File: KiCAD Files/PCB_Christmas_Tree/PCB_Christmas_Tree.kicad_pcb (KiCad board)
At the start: 2 copper layers, 129.4 x 60.1 mm, 67 parts, among them J1 Conn_01x03_Pin, J2 CR2032, J3 Conn_01x04_Pin, J4 Conn_01x04_Pin, J5 Conn_01x04_Pin, J7 Conn_01x04_Pin, Q1 PMOS, Q2 PMOS, Q3 PMOS, Q4 NPN, Q5 PMOS, SW1 SW_Omron_B3FS, U1 ATtiny402-SS

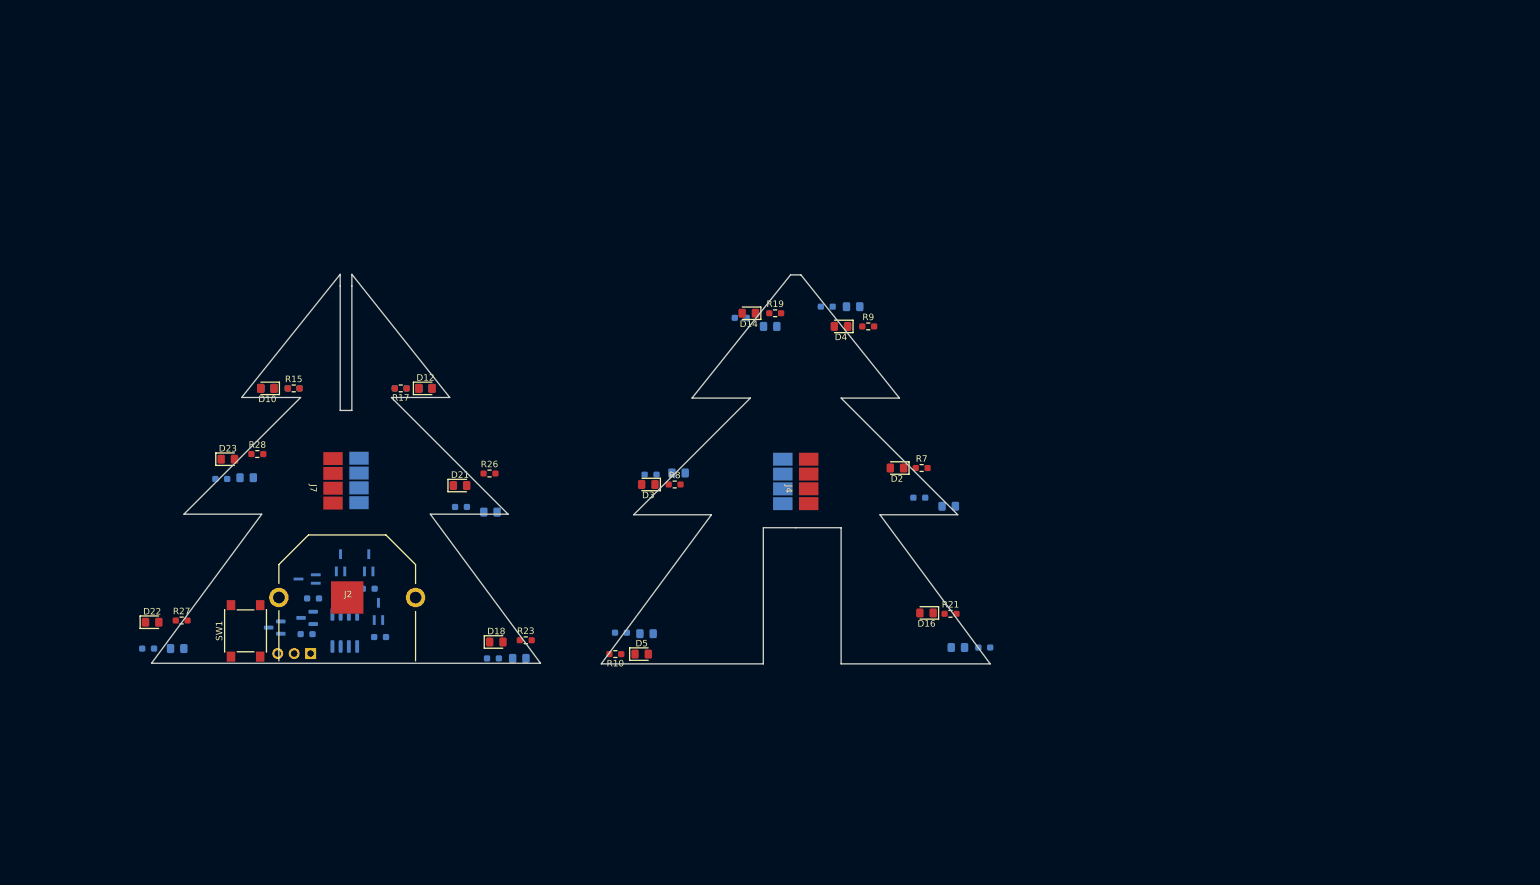
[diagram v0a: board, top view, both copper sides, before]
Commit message: pcb revision
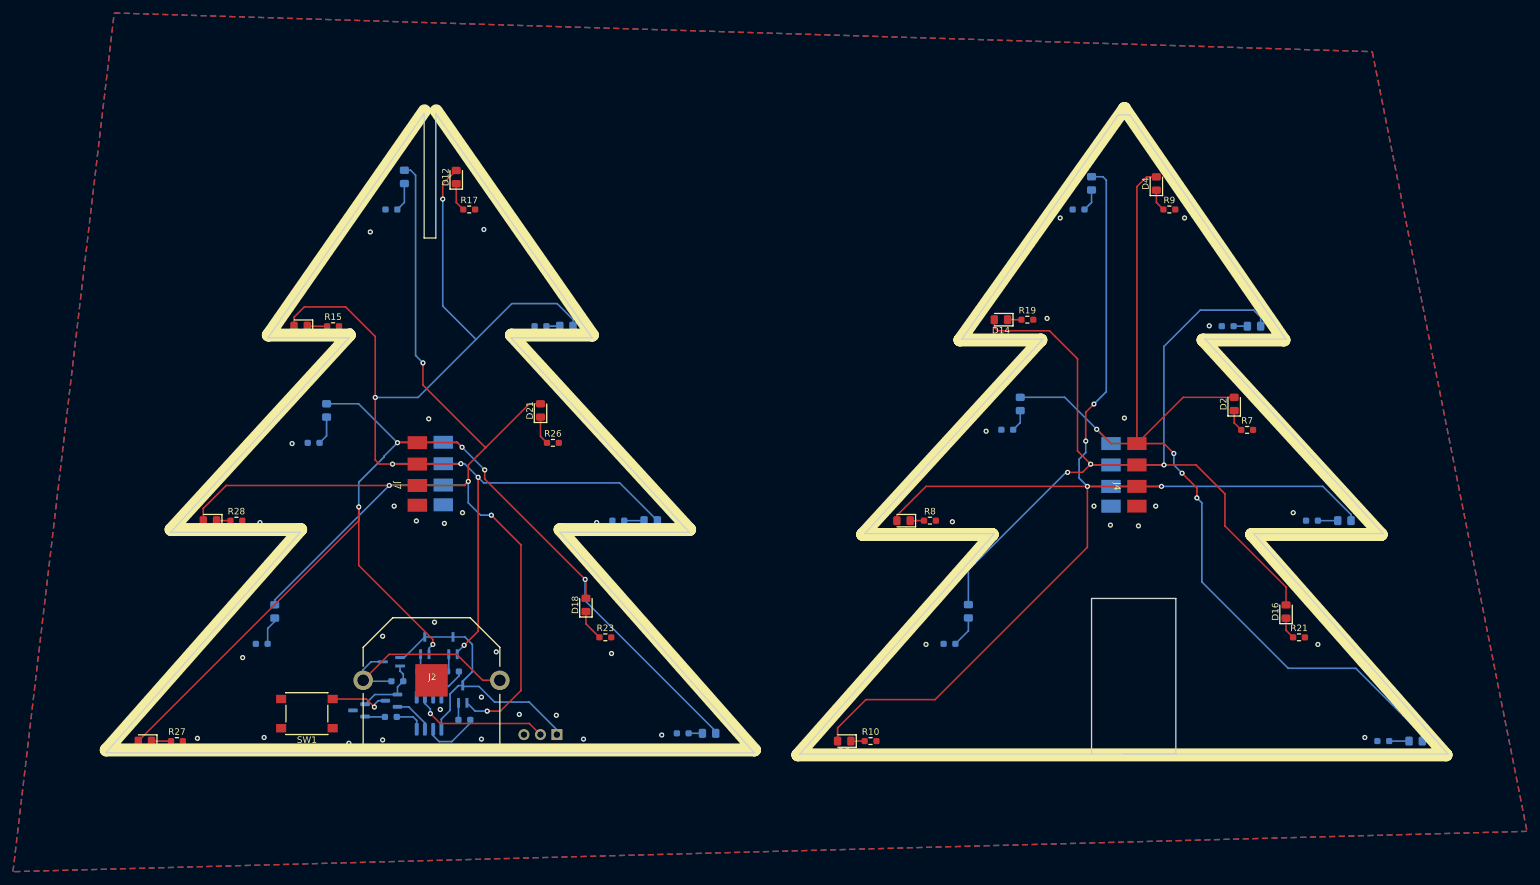
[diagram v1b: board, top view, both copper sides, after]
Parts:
- moved D11 72.1 mm to (248.0, 140.0), turned to 0 degrees
- moved R16 63.2 mm to (243.0, 140.0), turned to 180 degrees
- moved D15 61.9 mm to (223.1, 76.0)
- moved R20 61.9 mm to (219.0, 76.0)
- moved D24 61.1 mm to (237.0, 106.0), turned to 0 degrees
- moved R29 60.7 mm to (232.0, 106.0)
- moved R18 55.5 mm to (185.0, 92.0)
- moved D16 55.5 mm to (228.0, 120.0), turned to 90 degrees
- moved R25 54.7 mm to (196.0, 58.0)
- moved D20 54.3 mm to (198.0, 54.0), turned to 90 degrees
- moved R21 53.9 mm to (230.0, 124.0)
- moved D13 53.8 mm to (187.0, 88.0), turned to 90 degrees
- moved D4 53.4 mm to (208.0, 54.0), turned to 90 degrees
- moved D2 52.9 mm to (220.0, 88.0), turned to 90 degrees
- moved R22 50.7 mm to (176.1, 125.0)
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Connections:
- U1 pad 3: /LED_Set_3 -> /Switch_in
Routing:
- net /LED_Power_3: track 0.00 -> 395.9 mm, vias 0 -> 9
- net /LED_Power_2: track 0.00 -> 346.2 mm, vias 0 -> 9
- net /LED_Power_1: track 0.00 -> 346.0 mm, vias 0 -> 10
- net VDD: track 0.00 -> 46.5 mm
- net +BATT: track 0.00 -> 34.0 mm
- net /UDPI: track 0.00 -> 21.2 mm, vias 0 -> 1
- net Net-(Q1-G): track 0.00 -> 10.6 mm
- net Net-(D1-K): track 0.00 -> 9.27 mm, vias 0 -> 1
- net /LED_Set_3: track 0.00 -> 8.77 mm
- net /LED_Set_2: track 0.00 -> 6.80 mm
- net /Switch_in: track 0.00 -> 6.24 mm
- net Net-(D18-K): track 0.00 -> 4.84 mm
- net Net-(D17-K): track 0.00 -> 4.83 mm
- net /LED_Set_1: track 0.00 -> 4.83 mm
- net /Power_sustain: track 0.00 -> 4.66 mm
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- added copper zone on B.Cu, net GND
- added copper zone on F.Cu, net GND
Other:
- board size 129.4 x 60.1 mm -> 207.1 x 98.8 mm
